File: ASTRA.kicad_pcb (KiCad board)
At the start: 2 copper layers, 98.5 x 87.4 mm, 37 parts, among them M1 NEMA17, M2 NEMA17, P1 12V-DC, SW1 TOP, SW2 BOTTOM, SW3 LEFT, SW4 RIGHT, SW5 SELECT, SW6 RETURN, SW7 RESET, T1 TMC2209, T2 TMC2209, U1 MCP23017x-x-SP

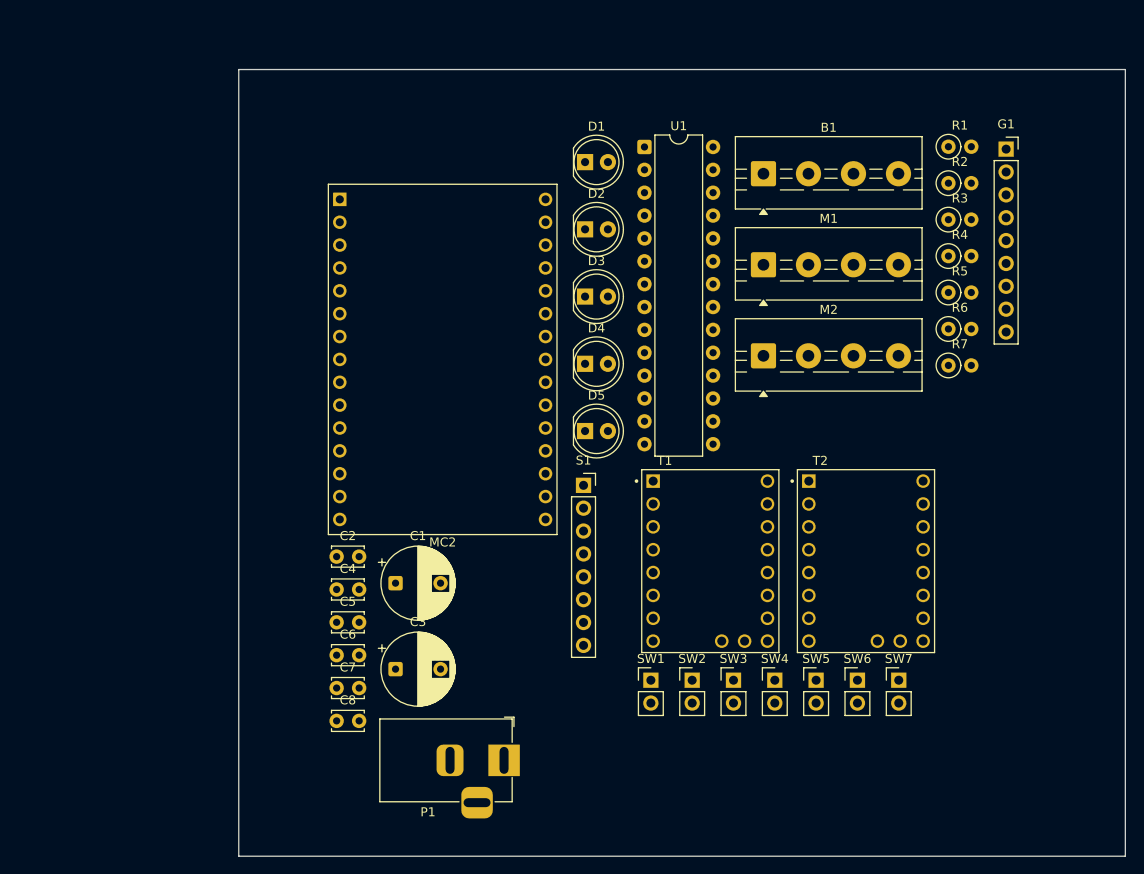
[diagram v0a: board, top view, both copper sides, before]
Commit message: V3 finished schem
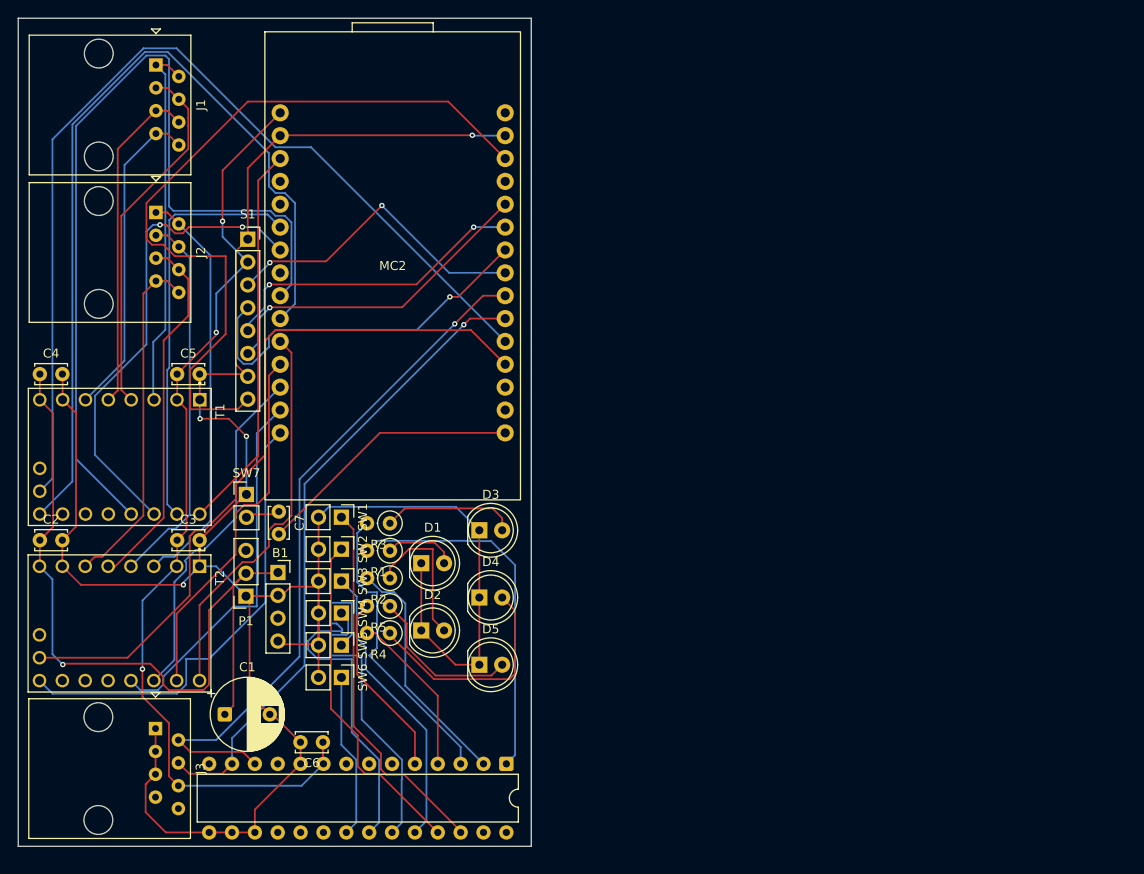
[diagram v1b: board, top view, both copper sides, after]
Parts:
- removed C8: 100nF, Capacitor_THT:C_Disc_D3.4mm_W2.1mm_P2.50mm
- removed G1: BNO085, Connector_PinSocket_2.54mm:PinSocket_1x09_P2.54mm_Vertical
- removed M1, M2: NEMA17, TerminalBlock:TerminalBlock_MaiXu_MX126-5.0-04P_1x04_P5.00mm
- removed R6, R7: 4.7kR, Resistor_THT:R_Axial_DIN0207_L6.3mm_D2.5mm_P2.54mm_Vertical
- added J1: RJ45 (NEMA 17), Connector_RJ:RJ45_Amphenol_54602-x08_Horizontal, F.Cu at (88.0, 55.1)
- added J2: RJ45 (NEMA 17), Connector_RJ:RJ45_Amphenol_54602-x08_Horizontal, F.Cu at (88.0, 71.5)
- added J3: RJ45 (BNO085), Connector_RJ:RJ45_Amphenol_54602-x08_Horizontal, F.Cu at (88.0, 128.8)
- B1: footprint TerminalBlock:TerminalBlock_MaiXu_MX126-5.0-04P_1x04_P5.00mm -> Connector_PinSocket_2.54mm:PinSocket_1x04_P2.54mm_Vertical
- C3: value 680uF -> 100nF; footprint Capacitor_THT:CP_Radial_D8.0mm_P5.00mm -> Capacitor_THT:C_Disc_D3.4mm_W2.1mm_P2.50mm
- MC2: footprint RF_Module:ESP32-C3-DevKitM-1 -> ASTRAfootprints:ESP32-WROOM-32D-Devkit
- P1: footprint Connector_BarrelJack:BarrelJack_Horizontal -> Connector_PinSocket_2.54mm:PinSocket_1x03_P2.54mm_Vertical
- moved T2 83.2 mm to (84.0, 117.1), turned to -90 degrees
- moved R1 76.6 mm to (114.0, 109.1), turned to 180 degrees
- moved R2 76.0 mm to (114.1, 112.1), turned to 180 degrees
- moved SW7 75.4 mm to (98.1, 102.8)
- moved R4 74.9 mm to (114.0, 118.2), turned to 180 degrees
- moved R5 71.2 mm to (114.0, 115.2), turned to 180 degrees
- moved R3 70.6 mm to (114.0, 106.0), turned to 180 degrees
- moved U1 70.2 mm to (127.0, 132.7), turned to -90 degrees
- moved B1 69.8 mm to (101.6, 111.5)
- moved T1 66.6 mm to (84.0, 98.6), turned to -90 degrees
- moved SW6 57.3 mm to (108.7, 123.1), turned to -90 degrees
- moved SW5 52.9 mm to (108.6, 119.6), turned to -90 degrees
- moved SW4 48.7 mm to (108.7, 116.0), turned to -90 degrees
- moved D1 48.1 mm to (117.5, 110.4)
- moved D2 48.1 mm to (117.5, 117.9)
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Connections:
- B1 pad 2: +12V -> GND
- B1 pad 3: +12V -> +5V
- B1 pad 4: +12V -> GND
- C1 pad 2: +12V -> GND
- C2 pad 2: +12V -> GND
- C3 pad 1: +12V -> +3.3V
- C3 pad 2: +12V -> GND
- C4 pad 2: +12V -> GND
- C5 pad 2: +12V -> GND
- C6 pad 2: +12V -> GND
- C7 pad 1: +3.3V -> Net-(C7-Pad1)
- C7 pad 2: +12V -> Net-(MC2-Pin_30)
- D1 pad 1: +12V -> GND
- D2 pad 1: +12V -> GND
- D3 pad 1: +12V -> GND
- D4 pad 1: +12V -> GND
- D5 pad 1: +12V -> GND
- MC2 pad 1: Net-(MC2-Pin_1) -> +3.3V
- MC2 pad 10: /RES -> /2EN
- MC2 pad 11: /MOSI -> /1DIR
- MC2 pad 12: unconnected-(MC2-Pin_23-Pad12) -> /1STEP
- MC2 pad 13: /SCK -> /1PDN
- MC2 pad 14: +12V -> /1UART
- MC2 pad 15: unconnected-(MC2-Pin_29-Pad15) -> /1EN
- MC2 pad 16: +3.3V -> Net-(MC2-Pin_30)
- MC2 pad 17: +12V -> unconnected-(MC2-Pin_28-Pad17)
- MC2 pad 19: unconnected-(MC2-Pin_24-Pad19) -> /T2_DIAG
- MC2 pad 2: unconnected-(MC2-Pin_3-Pad2) -> GND
- MC2 pad 20: unconnected-(MC2-Pin_22-Pad20) -> /T1_DIAG
- MC2 pad 21: Net-(MC2-Pin_20) -> /SDA
- MC2 pad 22: Net-(MC2-Pin_18) -> /SCL
- MC2 pad 23: Net-(MC2-Pin_16) -> /SCK
- MC2 pad 24: Net-(MC2-Pin_14) -> /MOSI
- MC2 pad 25: Net-(MC2-Pin_12) -> /RES
- MC2 pad 26: Net-(MC2-Pin_10) -> /DC
- MC2 pad 27: Net-(MC2-Pin_8) -> unconnected-(MC2-Pin_8-Pad27)
- MC2 pad 28: Net-(MC2-Pin_6) -> /BL
- MC2 pad 29: Net-(MC2-Pin_4) -> GND
- MC2 pad 3: unconnected-(MC2-Pin_5-Pad3) -> /2DIR
- MC2 pad 30: Net-(MC2-Pin_2) -> unconnected-(MC2-Pin_2-Pad30)
- MC2 pad 4: /T2_DIAG -> unconnected-(MC2-Pin_7-Pad4)
- MC2 pad 5: /T1_DIAG -> unconnected-(MC2-Pad5)
- MC2 pad 6: /SDA -> /2STEP
- MC2 pad 7: /SCL -> /2PDN
- MC2 pad 8: /BL -> unconnected-(MC2-Pin_15-Pad8)
- MC2 pad 9: /DC -> /2UART
- P1 pad 1: +12V -> GND
- R1 pad 2: Net-(U1-GPA0) -> Net-(U1-GPB0)
- R2 pad 2: Net-(U1-GPA1) -> Net-(U1-GPB1)
- R3 pad 2: Net-(U1-GPA2) -> Net-(U1-GPB2)
- R4 pad 2: Net-(U1-GPA3) -> Net-(U1-GPB3)
- R5 pad 2: Net-(U1-GPA4) -> Net-(U1-GPB4)
- S1 pad 1: +12V -> GND
- S1 pad 7: +12V -> GND
- SW1 pad 1: Net-(U1-GPB0) -> Net-(U1-GPA5)
- SW1 pad 2: +12V -> GND
- SW2 pad 1: Net-(U1-GPB1) -> Net-(U1-GPA4)
- SW2 pad 2: +12V -> GND
- SW3 pad 1: Net-(U1-GPB2) -> Net-(U1-GPA3)
- SW3 pad 2: +12V -> GND
- SW4 pad 1: Net-(U1-GPB3) -> Net-(U1-GPA2)
- SW4 pad 2: +12V -> GND
- SW5 pad 1: Net-(U1-GPB4) -> Net-(U1-GPA1)
- SW5 pad 2: +12V -> GND
- SW6 pad 1: Net-(U1-GPB5) -> Net-(U1-GPA0)
- SW6 pad 2: +12V -> GND
- SW7 pad 1: unconnected-(SW7-Pad1) -> GND
- SW7 pad 2: Net-(C8-Pad1) -> Net-(C7-Pad1)
- T1 pad 1: +12V -> GND
- T1 pad 10: Net-(MC2-Pin_14) -> /2STEP
- T1 pad 11: Net-(MC2-Pin_18) -> /2PDN
- T1 pad 12: Net-(MC2-Pin_20) -> /2UART
- T1 pad 16: Net-(MC2-Pin_12) -> /2EN
- T1 pad 7: +12V -> GND
- T1 pad 9: Net-(MC2-Pin_16) -> /2DIR
- T2 pad 1: +12V -> GND
- T2 pad 10: Net-(MC2-Pin_4) -> /1STEP
- T2 pad 11: Net-(MC2-Pin_8) -> /1PDN
- T2 pad 12: Net-(MC2-Pin_10) -> /1UART
- T2 pad 16: Net-(MC2-Pin_2) -> /1EN
- T2 pad 7: +12V -> GND
- T2 pad 9: Net-(MC2-Pin_6) -> /1DIR
- U1 pad 10: +12V -> GND
- U1 pad 12: Net-(U1-SCK) -> /SCL
- U1 pad 13: Net-(U1-SDA) -> /SDA
- U1 pad 15: +12V -> GND
- U1 pad 16: +12V -> GND
- U1 pad 17: +12V -> GND
- U1 pad 26: unconnected-(U1-GPA5-Pad26) -> Net-(U1-GPA5)
- U1 pad 6: Net-(U1-GPB5) -> unconnected-(U1-GPB5-Pad6)
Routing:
- net GND: track 0.00 -> 273.8 mm, vias 0 -> 4
- net /T1_DIAG: track 0.00 -> 107.6 mm
- net +3.3V: track 0.00 -> 105.5 mm, vias 0 -> 3
- net /2UART: track 0.00 -> 98.8 mm
- net /2EN: track 0.00 -> 95.5 mm
- net +12V: track 0.00 -> 87.2 mm, vias 0 -> 1
- net /BL: track 0.00 -> 86.3 mm
- net /T2_DIAG: track 0.00 -> 80.7 mm
- net /SCL: track 0.00 -> 77.9 mm, vias 0 -> 1
- net /SDA: track 0.00 -> 71.3 mm, vias 0 -> 1
- net /2PDN: track 0.00 -> 53.4 mm, vias 0 -> 2
- net /1EN: track 0.00 -> 51.1 mm
- net /2STEP: track 0.00 -> 46.4 mm
- net Net-(T2-M1B): track 0.00 -> 46.3 mm
- net /1DIR: track 0.00 -> 43.7 mm
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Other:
- board size 98.5 x 87.4 mm -> 57 x 92 mm
